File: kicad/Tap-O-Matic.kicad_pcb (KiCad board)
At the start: 2 copper layers, 120.7 x 108 mm, 64 parts, among them J1 fuzzySI_thonkiconn, J16 Conn_02x05_Odd_Even, J2 fuzzySI_thonkiconn, J3 fuzzySI_thonkiconn, J4 fuzzySI_thonkiconn, J5 fuzzySI_thonkiconn, J6 fuzzySI_thonkiconn, J7 fuzzySI_thonkiconn, J8 fuzzySI_thonkiconn, J9 fuzzySI_thonkiconn, SW1 SW_SPDT, SW2 SW_SPDT, U1 DaisySubmodule, U2 4051, U3 4051, U4 4051, U5 DG408

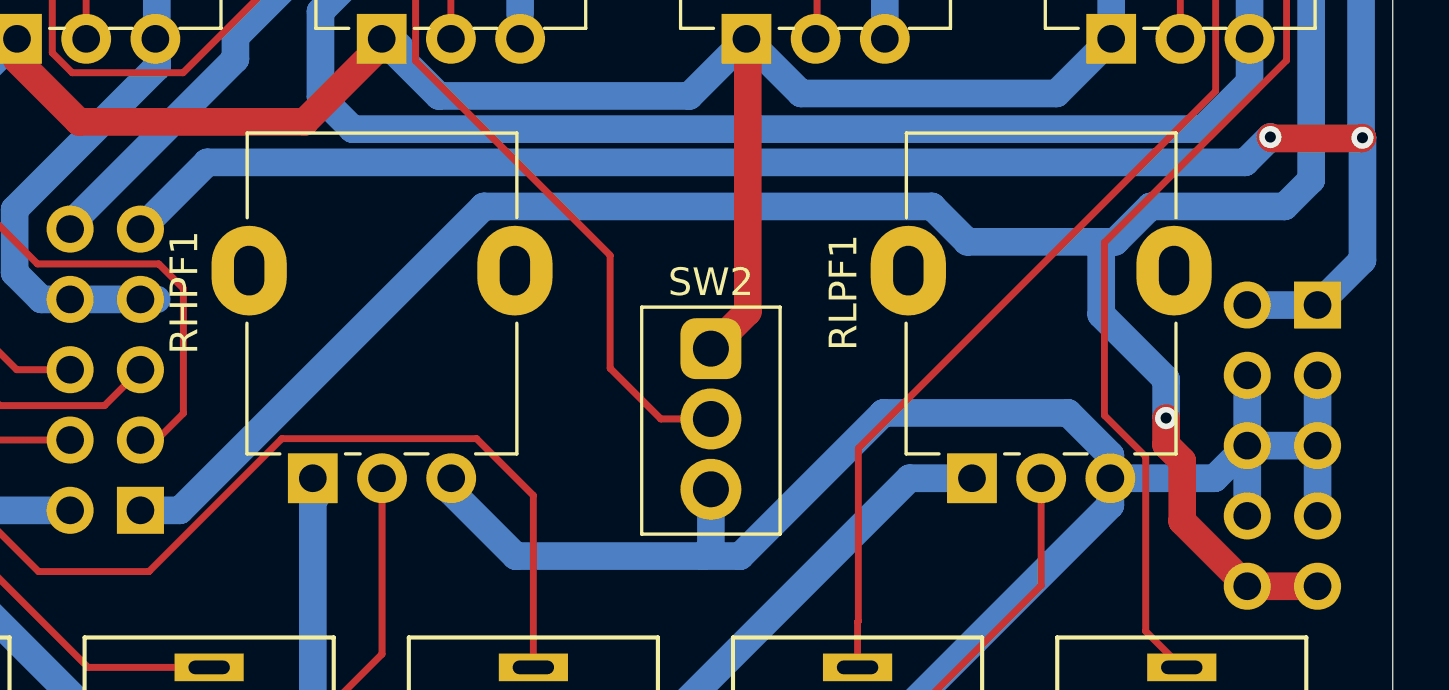
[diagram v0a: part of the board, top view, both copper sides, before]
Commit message: full changes for second iteration
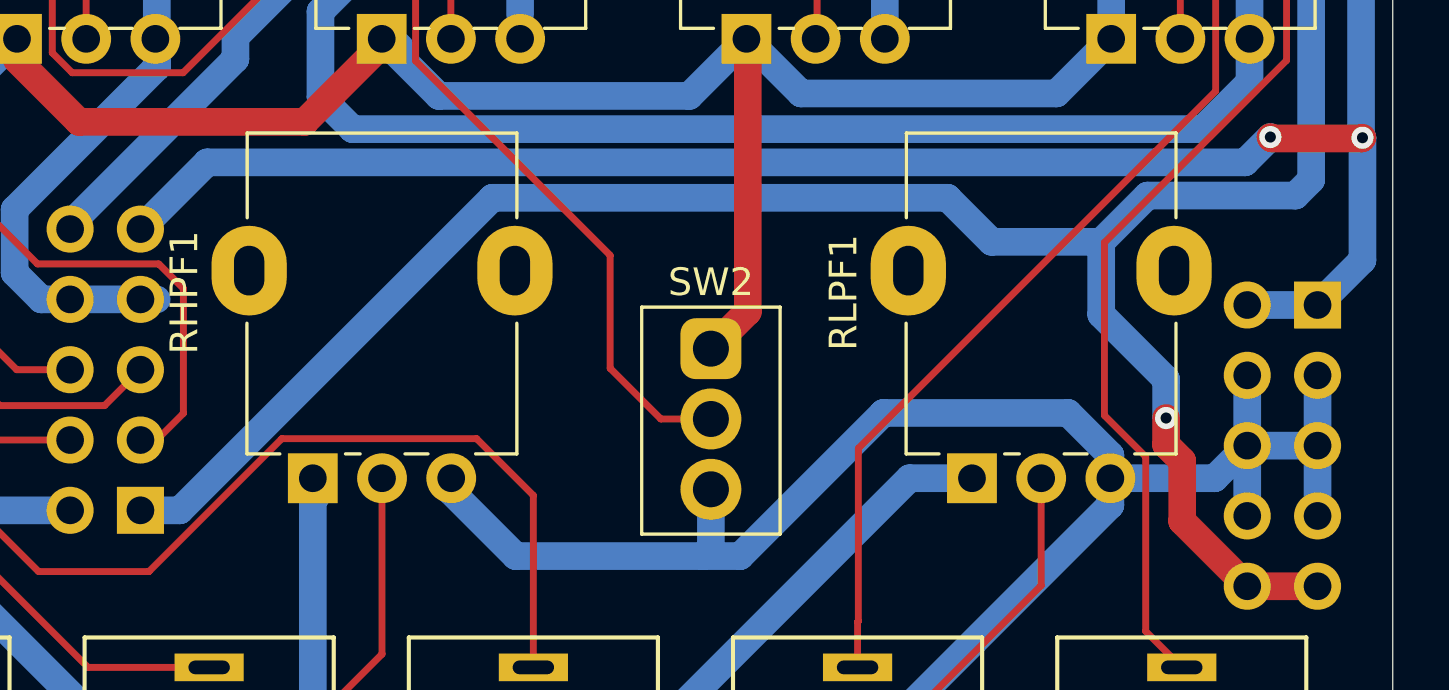
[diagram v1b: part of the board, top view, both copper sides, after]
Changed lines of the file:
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@@
 		(pad_to_mask_clearance 0)
 		(allow_soldermask_bridges_in_footprints no)
-		(grid_origin 18.542 16.891)
+		(grid_origin 0 -107.95)
 		(pcbplotparams
 			(layerselection 0x00010fc_ffffffff)
@@
 	(segment
 		(start 110.119414 -28.294752)
+		(end 106.160837 -28.294752)
+		(width 1)
+		(layer "B.Cu")
+		(net 19)
+	)
+	(segment
+		(start 110.119414 -28.294752)
 		(end 110.119414 -25.669777)
 		(width 1)
@@
 	)
 	(segment
-		(start 87.81578 -29.57358)
-		(end 76.837 -18.5948)
+		(start 76.837 -18.5948)
+		(end 75.41 -18.5948)
 		(width 1)
 		(layer "B.Cu")
@@
 	)
 	(segment
-		(start 117.7036 -30.5308)
-		(end 117.677626 -30.504826)
+		(start 117.138367 -29.965567)
+		(end 111.790229 -29.965567)
 		(width 1)
 		(layer "B.Cu")
@@
 	)
 	(segment
-		(start 117.7036 -30.5308)
-		(end 116.74638 -29.57358)
-		(width 1)
-		(layer "B.Cu")
-		(net 19)
-	)
-	(segment
-		(start 105.282748 -28.294752)
-		(end 104.00392 -29.57358)
+		(start 108.966 -72.9488)
+		(end 108.966 -64.8208)
 		(width 1)
 		(layer "B.Cu")
@@
 	)
 	(segment
-		(start 108.966 -72.9488)
-		(end 108.966 -64.8208)
+		(start 106.160837 -28.294752)
+		(end 104.569707 -29.885882)
 		(width 1)
 		(layer "B.Cu")
@@
 	)
 	(segment
-		(start 76.837 -18.5948)
-		(end 75.41 -18.5948)
+		(start 111.790229 -29.965567)
+		(end 110.119414 -28.294752)
 		(width 1)
 		(layer "B.Cu")
@@
 	)
 	(segment
-		(start 110.618532 -28.294752)
-		(end 110.119414 -28.294752)
+		(start 88.128082 -29.885882)
+		(end 76.837 -18.5948)
 		(width 1)
 		(layer "B.Cu")
@@
 	)
 	(segment
-		(start 116.74638 -29.57358)
-		(end 111.89736 -29.57358)
+		(start 112.463862 -23.325329)
+		(end 112.463862 -21.929196)
 		(width 1)
 		(layer "B.Cu")
@@
 	)
 	(segment
-		(start 112.463862 -23.325329)
-		(end 112.463862 -21.929196)
+		(start 117.7036 -30.5308)
+		(end 117.138367 -29.965567)
 		(width 1)
 		(layer "B.Cu")
@@
 	)
 	(segment
-		(start 111.89736 -29.57358)
-		(end 110.618532 -28.294752)
-		(width 1)
-		(layer "B.Cu")
-		(net 19)
-	)
-	(segment
-		(start 110.119414 -28.294752)
-		(end 105.282748 -28.294752)
-		(width 1)
-		(layer "B.Cu")
-		(net 19)
-	)
-	(segment
-		(start 104.00392 -29.57358)
-		(end 87.81578 -29.57358)
+		(start 104.569707 -29.885882)
+		(end 88.128082 -29.885882)
 		(width 1)
 		(layer "B.Cu")
